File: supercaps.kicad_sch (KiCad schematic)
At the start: 21 parts, among them J8 XT30_F, J9 XT30_F, Q10 2SAR587D3, Q9 2SCR587D3, U17 TLV9301xDBV

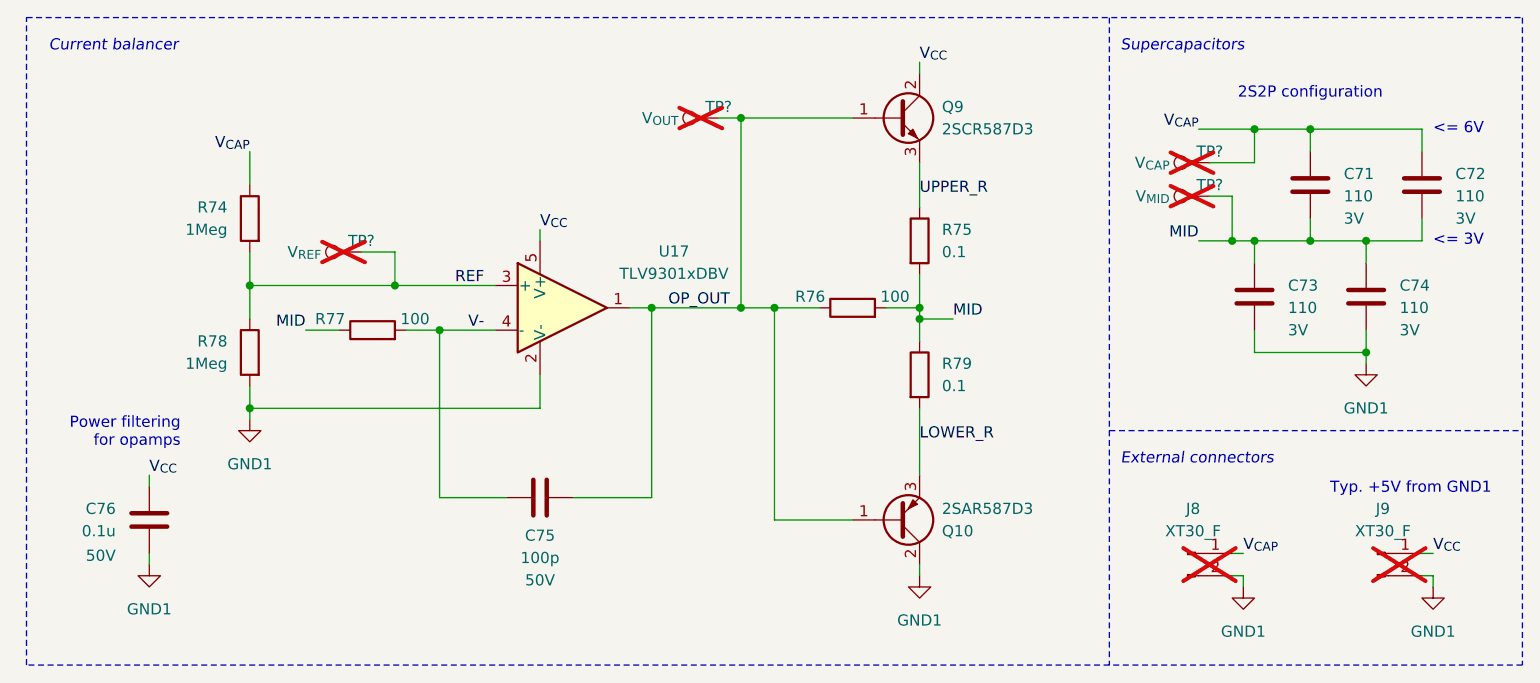
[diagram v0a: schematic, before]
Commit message: Unsure of changes
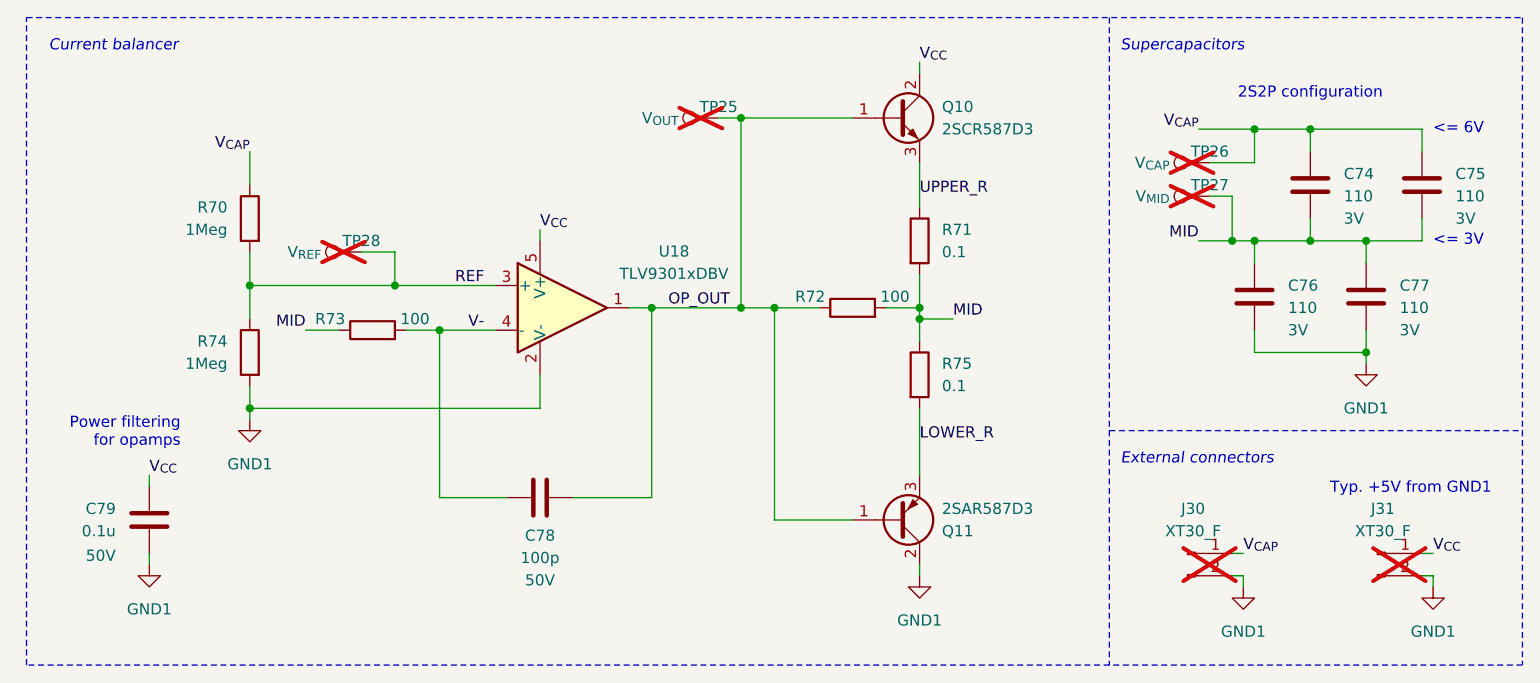
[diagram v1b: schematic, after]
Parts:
- gave numbers to parts that had none: 4
- renumbered C71 to C74, C72 to C75, C73 to C76, C74 to C77, C75 to C78, C76 to C79, J8 to J30, J9 to J31, Q9 to Q10, Q10 to Q11, R74 to R70, R75 to R71, R76 to R72, R77 to R73, R78 to R74, R79 to R75, U17 to U18
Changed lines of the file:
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@@
 		(on_board yes)
 		(dnp yes)
-		(property "Reference" "TP?"
+		(property "Reference" "TP28"
 			(at 59.69 50.8 90)
 			(effects
@@
 		)
 		(instances
-			(project "SupercapManager"
-				(path "/6197145b-e7d4-44cc-9d90-537b6501bf60/e69614f9-5cd8-4aa3-ae42-53f80cb78886"
-					(reference "TP?")
-					(unit 1)
-				)
-			)
 			(project "Rev 1B"
 				(path "/e5f99deb-ef42-4c5f-b80a-388477910e20/1165d5b5-e274-4083-890a-7a12aee56ddf"
@@
 		(on_board yes)
 		(dnp no)
-		(property "Reference" "R79"
+		(property "Reference" "R75"
 			(at 125.73 64.7699 0)
 			(effects
@@
 		(on_board yes)
 		(dnp no)
-		(property "Reference" "U17"
+		(property "Reference" "U18"
 			(at 95.25 51.9998 0)
 			(effects
@@
 		(on_board yes)
 		(dnp yes)
-		(property "Reference" "TP?"
+		(property "Reference" "TP25"
 			(at 100.33 35.56 90)
 			(effects
@@
 		)
 		(instances
-			(project "SupercapManager"
-				(path "/6197145b-e7d4-44cc-9d90-537b6501bf60/e69614f9-5cd8-4aa3-ae42-53f80cb78886"
-					(reference "TP?")
-					(unit 1)
-				)
-			)
 			(project "Rev 1B"
 				(path "/e5f99deb-ef42-4c5f-b80a-388477910e20/1165d5b5-e274-4083-890a-7a12aee56ddf"
@@
 		(on_board yes)
 		(dnp no)
-		(property "Reference" "C75"
+		(property "Reference" "C78"
 			(at 80.01 84.328 90)
 			(effects
@@
 		(on_board yes)
 		(dnp no)
-		(property "Reference" "C73"
+		(property "Reference" "C76"
 			(at 165.1 55.8799 0)
 			(effects
@@
 		(dnp no)
 		(fields_autoplaced yes)
-		(property "Reference" "#PWR098"
+		(property "Reference" "#PWR0119"
 			(at 46.99 77.47 0)
 			(effects
@@
 		(on_board yes)
 		(dnp no)
-		(property "Reference" "C76"
+		(property "Reference" "C79"
 			(at 31.75 81.2799 0)
 			(effects
@@
 		(dnp no)
 		(fields_autoplaced yes)
-		(property "Reference" "#PWR0101"
+		(property "Reference" "#PWR0122"
 			(at 160.02 96.52 0)
 			(effects
@@
 		(on_board yes)
 		(dnp yes)
-		(property "Reference" "J9"
+		(property "Reference" "J31"
 			(at 175.895 81.28 0)
 			(effects
@@
 		(dnp no)
 		(fields_autoplaced yes)
-		(property "Reference" "#PWR097"
+		(property "Reference" "#PWR0118"
 			(at 173.99 71.12 0)
 			(effects
@@
 		(on_board yes)
 		(dnp yes)
-		(property "Reference" "TP?"
+		(property "Reference" "TP26"
 			(at 156.21 40.64 90)
 			(effects
@@
 		)
 		(instances
-			(project "SupercapManager"
-				(path "/6197145b-e7d4-44cc-9d90-537b6501bf60/e69614f9-5cd8-4aa3-ae42-53f80cb78886"
-					(reference "TP?")
-					(unit 1)
-				)
-			)
 			(project "Rev 1B"
 				(path "/e5f99deb-ef42-4c5f-b80a-388477910e20/1165d5b5-e274-4083-890a-7a12aee56ddf"
@@
 		(on_board yes)
 		(dnp no)
-		(property "Reference" "R74"
+		(property "Reference" "R70"
 			(at 44.45 46.9899 0)
 			(effects
@@
 		(on_board yes)
 		(dnp no)
-		(property "Reference" "C71"
+		(property "Reference" "C74"
 			(at 171.45 43.1799 0)
 			(effects
@@
 		(dnp no)
 		(fields_autoplaced yes)
-		(property "Reference" "#PWR0100"
+		(property "Reference" "#PWR0121"
 			(at 123.19 95.25 0)
 			(effects
@@
 		(on_board yes)
 		(dnp yes)
-		(property "Reference" "J8"
+		(property "Reference" "J30"
 			(at 154.305 81.28 0)
 			(effects
@@
 		(dnp no)
 		(fields_autoplaced yes)
-		(property "Reference" "Q9"
+		(property "Reference" "Q10"
 			(at 125.73 35.5599 0)
 			(effects
@@
 		(on_board yes)
 		(dnp yes)
-		(property "Reference" "TP?"
+		(property "Reference" "TP27"
 			(at 156.21 44.45 90)
 			(effects
@@
 		)
 		(instances
-			(project "SupercapManager"
-				(path "/6197145b-e7d4-44cc-9d90-537b6501bf60/e69614f9-5cd8-4aa3-ae42-53f80cb78886"
-					(reference "TP?")
-					(unit 1)
-				)
-			)
 			(project "Rev 1B"
 				(path "/e5f99deb-ef42-4c5f-b80a-388477910e20/1165d5b5-e274-4083-890a-7a12aee56ddf"
@@
 		(on_board yes)
 		(dnp no)
-		(property "Reference" "C72"
+		(property "Reference" "C75"
 			(at 184.15 43.1799 0)
 			(effects
@@
 		(on_board yes)
 		(dnp no)
-		(property "Reference" "R75"
+		(property "Reference" "R71"
 			(at 125.73 49.5299 0)
 			(effects
@@
 		(on_board yes)
 		(dnp no)
-		(property "Reference" "R78"
+		(property "Reference" "R74"
 			(at 44.45 62.2299 0)
 			(effects
@@
 		(on_board yes)
 		(dnp no)
-		(property "Reference" "R77"
+		(property "Reference" "R73"
 			(at 56.134 59.69 90)
 			(effects
@@
 		(dnp no)
 		(fields_autoplaced yes)
-		(property "Reference" "#PWR099"
+		(property "Reference" "#PWR0120"
 			(at 35.56 93.98 0)
 			(effects
@@
 		(dnp no)
 		(fields_autoplaced yes)
-		(property "Reference" "#PWR0102"
+		(property "Reference" "#PWR0123"
 			(at 181.61 96.52 0)
 			(effects
@@
 		(on_board yes)
 		(dnp no)
-		(property "Reference" "R76"
+		(property "Reference" "R72"
 			(at 110.744 57.15 90)
 			(effects
@@
 		(on_board yes)
 		(dnp no)
-		(property "Reference" "Q10"
+		(property "Reference" "Q11"
 			(at 125.73 83.8201 0)
 			(effects
@@
 		(on_board yes)
 		(dnp no)
-		(property "Reference" "C74"
+		(property "Reference" "C77"
 			(at 177.8 55.8799 0)
 			(effects
